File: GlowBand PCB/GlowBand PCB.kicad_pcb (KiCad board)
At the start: 2 copper layers, 44 x 34.5 mm, 74 parts, among them P1 Solder_Pad, P2 Solder_Pad, P3 Solder_Pad, P4 Solder_Pad, P5 Solder_Pad, P6 Solder_Pad, P7 Solder_Pad, P8 Solder_Pad, P9 Magnetic Pogopin 6pin female, SW1 TS24CA, SW2 TS24CA, SW3 TS-1185EC-C-D-B, SW4 TS-1185EC-C-D-B, U1 ESP32-WROOM-32E, U10 SN74LVC1G373DBVR, U13 AP40P05, U15 MSM261D4030H1CPM, U16 AP40P05, U17 AO3400A, U18 FS8205A, U19 TP4056, U2 FXL0530-6R8-M, U20 DW01A, U3 SN74LVC2T45DCUR, U4 TPS61032PWPR, U5 AP40P05, U6 SS54, U7 SPX3819M5-L-3-3_TR, U9 AP40P05

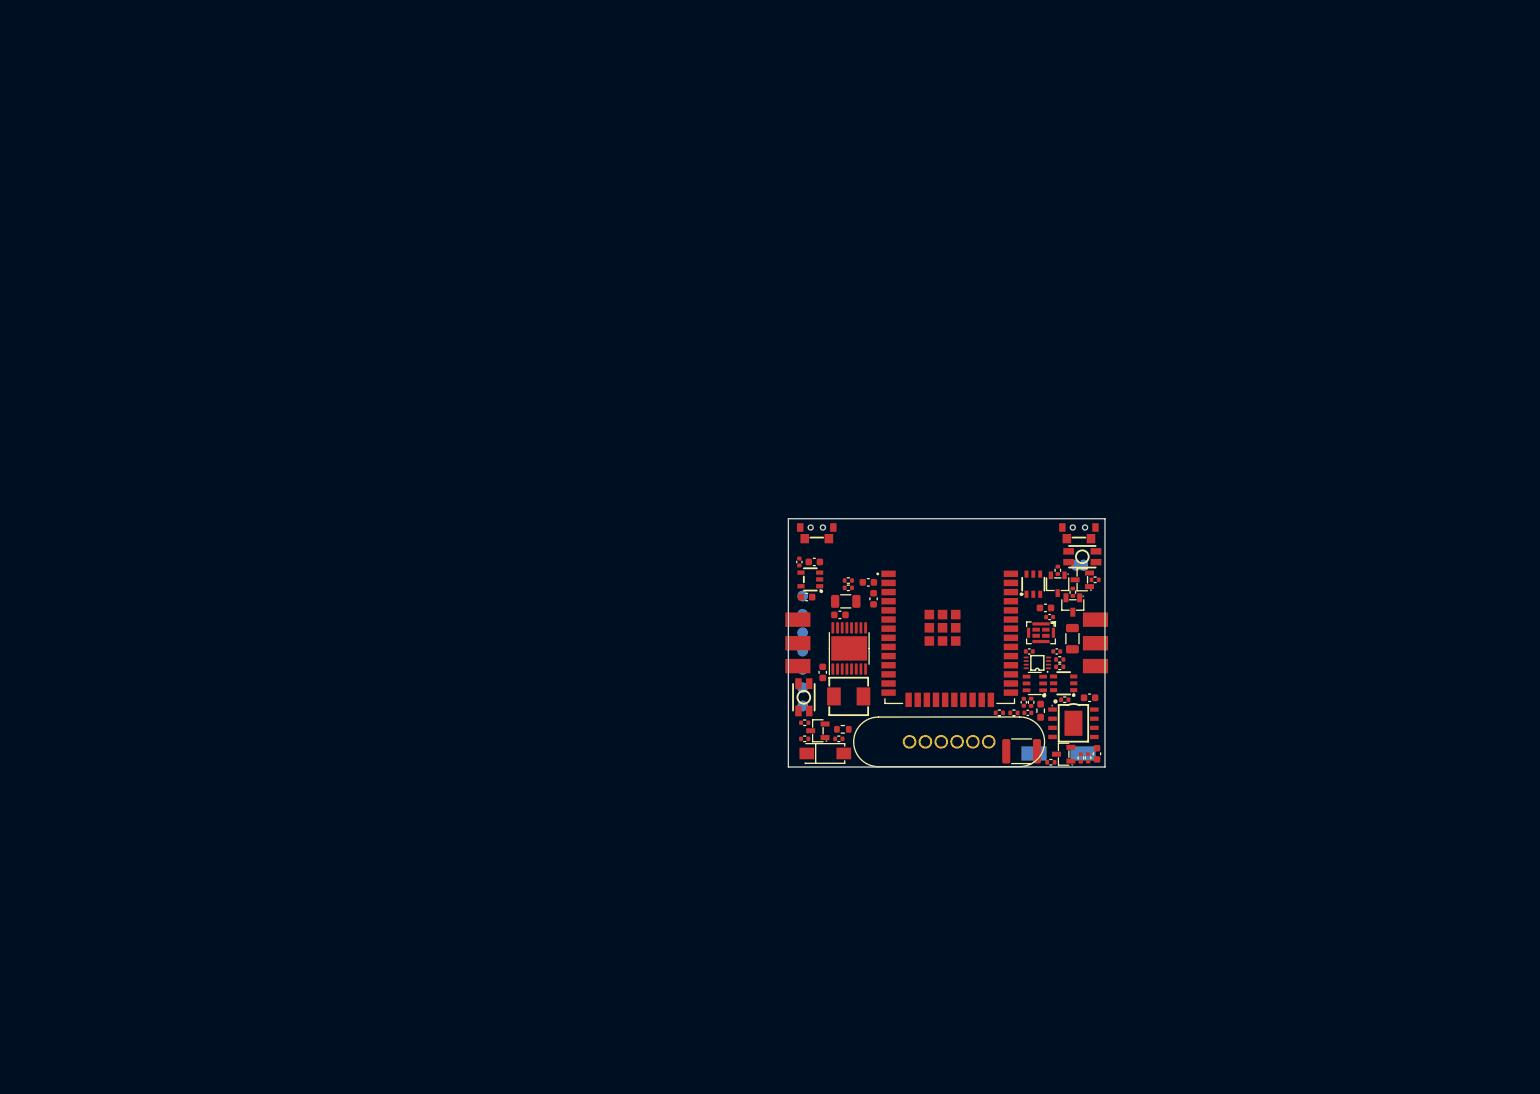
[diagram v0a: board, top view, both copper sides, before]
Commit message: updated pcbs
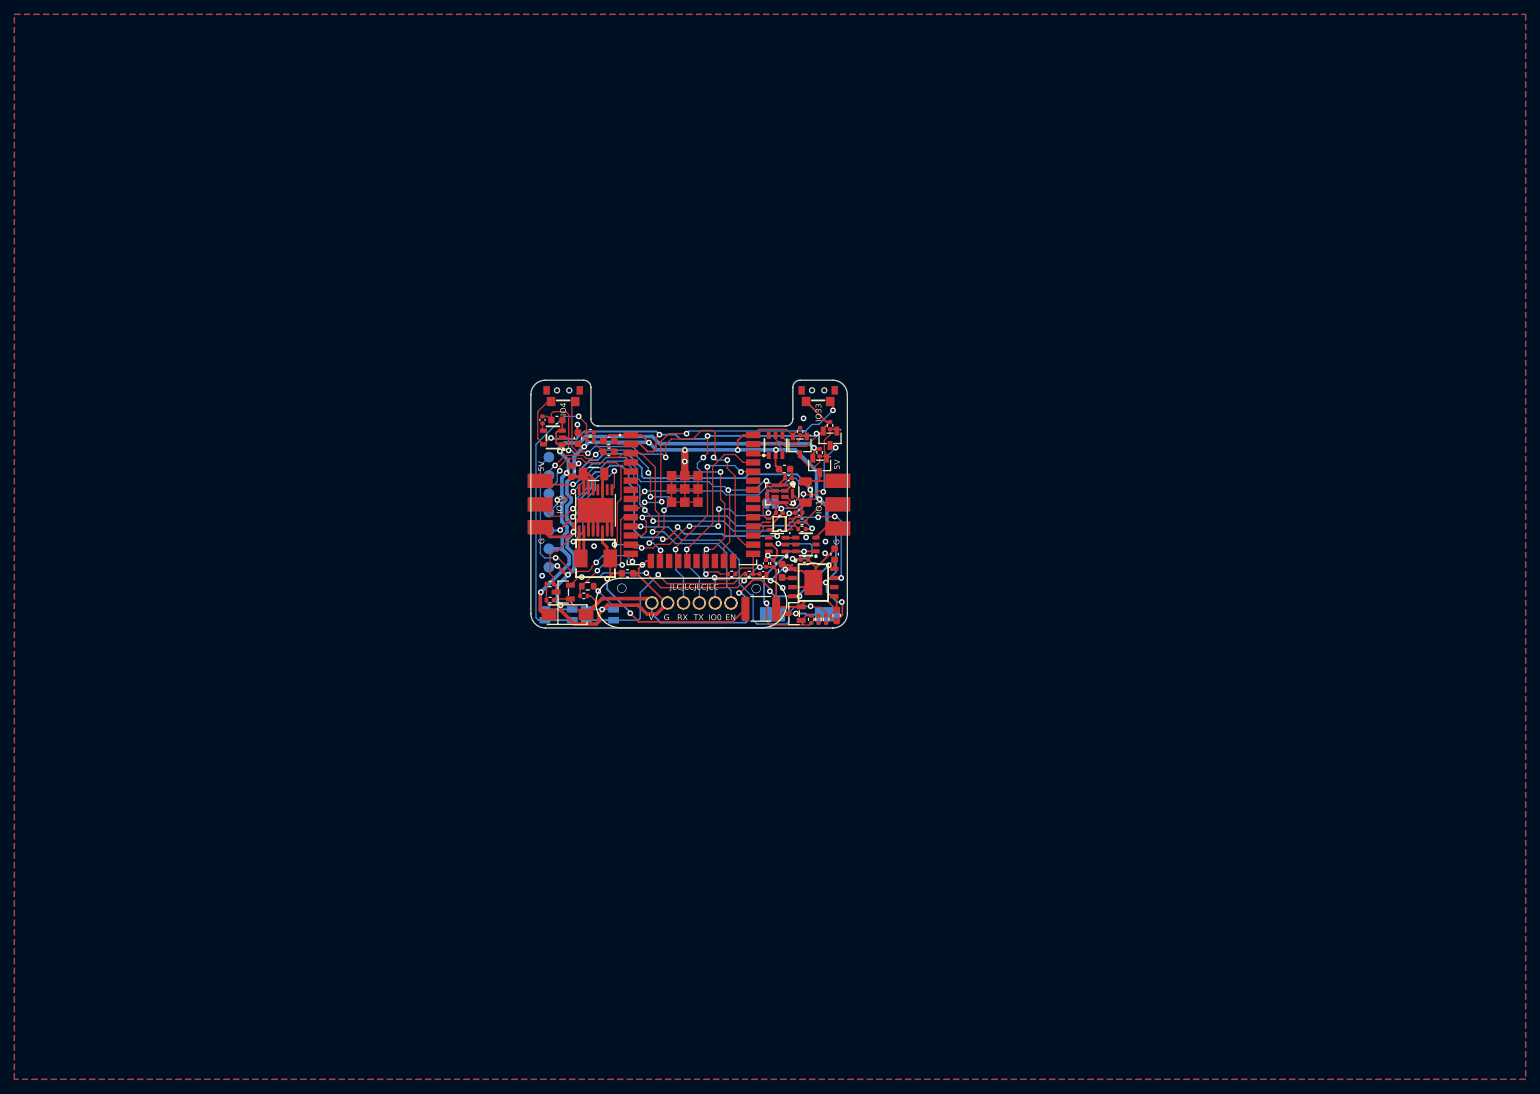
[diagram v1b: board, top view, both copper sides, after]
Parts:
- added G***: LOGO, LOGO, B.Cu at (93.6, 63.2)
- SW3, SW4: moved to B.Cu
- moved SW4 67.5 mm to (81.3, 83.4), turned to 180 degrees
- moved JP1 43.8 mm to (105.0, 67.8)
- moved R16 42.6 mm to (113.2, 57.0), turned to 90 degrees
- moved C12 42.3 mm to (109.8, 66.3)
- moved C5 42.3 mm to (77.3, 63.4), turned to -90 degrees
- moved U9 42.3 mm to (108.2, 83.2)
- moved C16 42.1 mm to (82.5, 60.7), turned to 180 degrees
- moved R21 41.9 mm to (99.6, 77.7)
- moved R19 41.5 mm to (102.0, 77.7)
- moved C17 41.5 mm to (103.9, 77.7)
- moved R18 41.4 mm to (79.9, 58.0)
- moved R20 41.4 mm to (79.9, 59.0)
- moved F1 41.3 mm to (103.6, 82.5)
- moved R13 41.2 mm to (111.6, 84.0), turned to -90 degrees
- moved R12 41.2 mm to (112.7, 84.0)
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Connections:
- SW1 pad 3: GND -> +3V3
- SW2 pad 3: GND -> +3V3
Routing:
- net GND: track 0.00 -> 287.0 mm, vias 0 -> 28
- net +3V3: track 0.00 -> 103.4 mm, vias 0 -> 9
- net +5V: track 0.00 -> 86.8 mm, vias 0 -> 4
- net 3.3V AFTER MOSFET: track 0.00 -> 69.7 mm, vias 0 -> 9
- net 5V AFTER MOSFET: track 0.00 -> 60.9 mm, vias 0 -> 3
- net VBUS: track 0.00 -> 57.6 mm, vias 0 -> 4
- net IO14/SCK/TMS: track 0.00 -> 55.4 mm, vias 0 -> 7
- net LED1 DATA OUT: track 0.00 -> 51.9 mm, vias 0 -> 4
- net +BATT: track 0.00 -> 51.2 mm, vias 0 -> 4
- net IO4/BUTTON2: track 0.00 -> 50.0 mm, vias 0 -> 4
- net IO15/WS/TDO: track 0.00 -> 49.8 mm, vias 0 -> 4
- net IO27/BATT CHARGING: track 0.00 -> 42.5 mm, vias 0 -> 4
- net IO26/BATT VOLT: track 0.00 -> 40.7 mm, vias 0 -> 2
- net IO33/MAINBUTTON: track 0.00 -> 40.5 mm, vias 0 -> 4
- net EN: track 0.00 -> 40.1 mm, vias 0 -> 1
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- added copper zone on B.Cu, net GND
- added copper zone on F.Cu, net GND
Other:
- board size 44 x 34.5 mm -> 44 x 34.4 mm
- board text added: "+ BATT"
- board text added: "- BATT"
- board text added: "3.3V OUT"
- board text added: "5V"
- board text added: "5V IN/OUT"
- board text added: "BOOT"
- board text added: "EN"
- board text added: "G"
- board text added: "GND"
- board text added: "GlowBand v1.0 beta 1"
- board text added: "IO0"
- board text added: "IO12/TDI"
- board text added: "IO13/TCK"
- board text added: "IO14/SCK/TMS"
- board text added: "IO15/WS/TDO"
- board text added: "IO16"
- board text added: "IO17"
- board text added: "IO33"
- board text added: "IO4"
- board text added: "JLCJLCJLCJLC"
- board text added: "Microphone on"
- board text added: "Place battery here. Make sure this PCB side is completely flat and cannot damage the battery."
- board text added: "RESET"
- board text added: "RX"
- board text added: "TX"
- board text added: "V"
- board text added: "https://bit.ly/ 3O7S2Tk"
